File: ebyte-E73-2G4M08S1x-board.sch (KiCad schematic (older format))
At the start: 39 parts, among them J1 USB_B_Micro, J2 USB_B_Micro, J3 BAT, J4 Conn_01x18_Male, J5 Conn_01x18_Male, J6 Conn_ARM_JTAG_SWD_10, J7 Conn_02x03_Odd_Even, Q1 PMV65XP, SW1 SW_Push, U1 MCP73831-2-OT, U2 LP5907MFX-3.3, U3 CH340E, U4 E73-2G4M08S1E, U5 L3GD20, Y1 Crystal

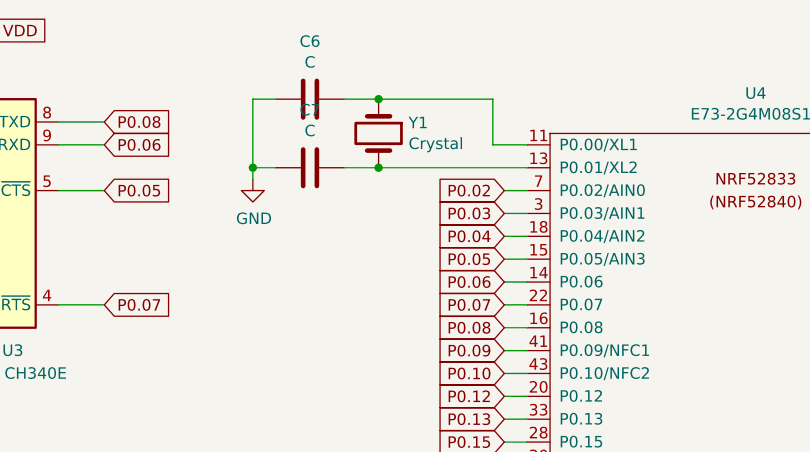
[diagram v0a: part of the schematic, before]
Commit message: Preliminary PCB layout
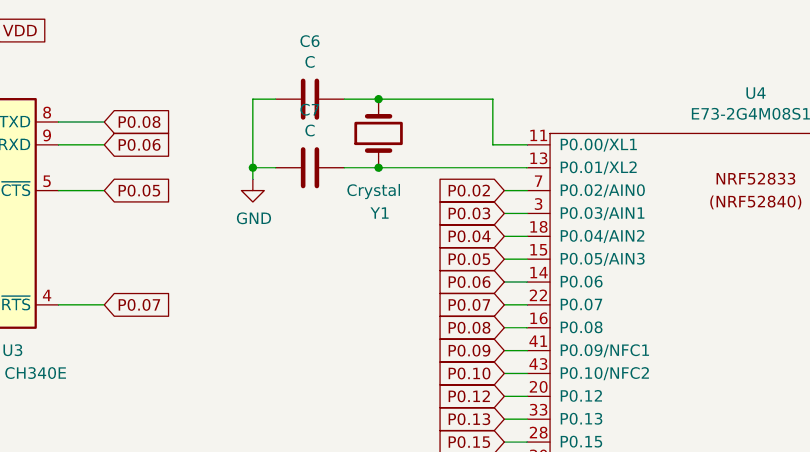
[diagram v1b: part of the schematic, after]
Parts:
- J1, J2: footprint Connector_USB:USB_Micro-AB_Molex_47590-0001 -> Connector_USB:USB_Micro-B_Amphenol_10103594-0001LF_Horizontal
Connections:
- net at C6.1, U4.11 (P0.00/XL1): now also Y1.2; no longer Y1.1
- net at C7.1, U4.13 (P0.01/XL2): now also Y1.1; no longer Y1.2
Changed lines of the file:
@@
 F 0 "J1" H 957 1867 50  0000 C CNN
 F 1 "USB_B_Micro" H 957 1776 50  0000 C CNN
-F 2 "Connector_USB:USB_Micro-AB_Molex_47590-0001" H 1050 1350 50  0001 C CNN
+F 2 "Connector_USB:USB_Micro-B_Amphenol_10103594-0001LF_Horizontal" H 1050 1350 50  0001 C CNN
 F 3 "~" H 1050 1350 50  0001 C CNN
 	1    900  1400
@@
 U 1 1 60519404
 P 4450 1150
-F 0 "Y1" V 4404 1281 50  0000 L CNN
-F 1 "Crystal" V 4495 1281 50  0000 L CNN
+F 0 "Y1" V 4100 1100 50  0000 L CNN
+F 1 "Crystal" V 4200 1050 50  0000 L CNN
 F 2 "Crystal:Crystal_SMD_MicroCrystal_MS3V-T1R" H 4450 1150 50  0001 C CNN
 F 3 "~" H 4450 1150 50  0001 C CNN
 	1    4450 1150
-	0    1    1    0
+	0    -1   -1   0
 $EndComp
 $Comp
@@
 F 0 "J2" H 957 3217 50  0000 C CNN
 F 1 "USB_B_Micro" H 957 3126 50  0000 C CNN
-F 2 "Connector_USB:USB_Micro-AB_Molex_47590-0001" H 1050 2700 50  0001 C CNN
+F 2 "Connector_USB:USB_Micro-B_Amphenol_10103594-0001LF_Horizontal" H 1050 2700 50  0001 C CNN
 F 3 "~" H 1050 2700 50  0001 C CNN
 	1    900  2750
